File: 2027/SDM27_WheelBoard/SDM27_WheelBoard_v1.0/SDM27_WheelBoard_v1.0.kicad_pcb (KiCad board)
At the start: 4 copper layers, 38 x 22 mm, 85 parts, among them IC1 TPS2121RUXR, IC2 TPS542951RSAR, IC3 TPS2121RUXR, IC4 MLX90614ESF-BAA-000-SP, IC5 SN74LVC1G17YZPR, IC8 TCAN3403DRBRQ1, J1 WEIPU SA12 7PIN, J2 WEIPU SA6 5Pin, U1 ESP32-C5, U2 USBLC6-2SC6, Y1 Crystal_GND24

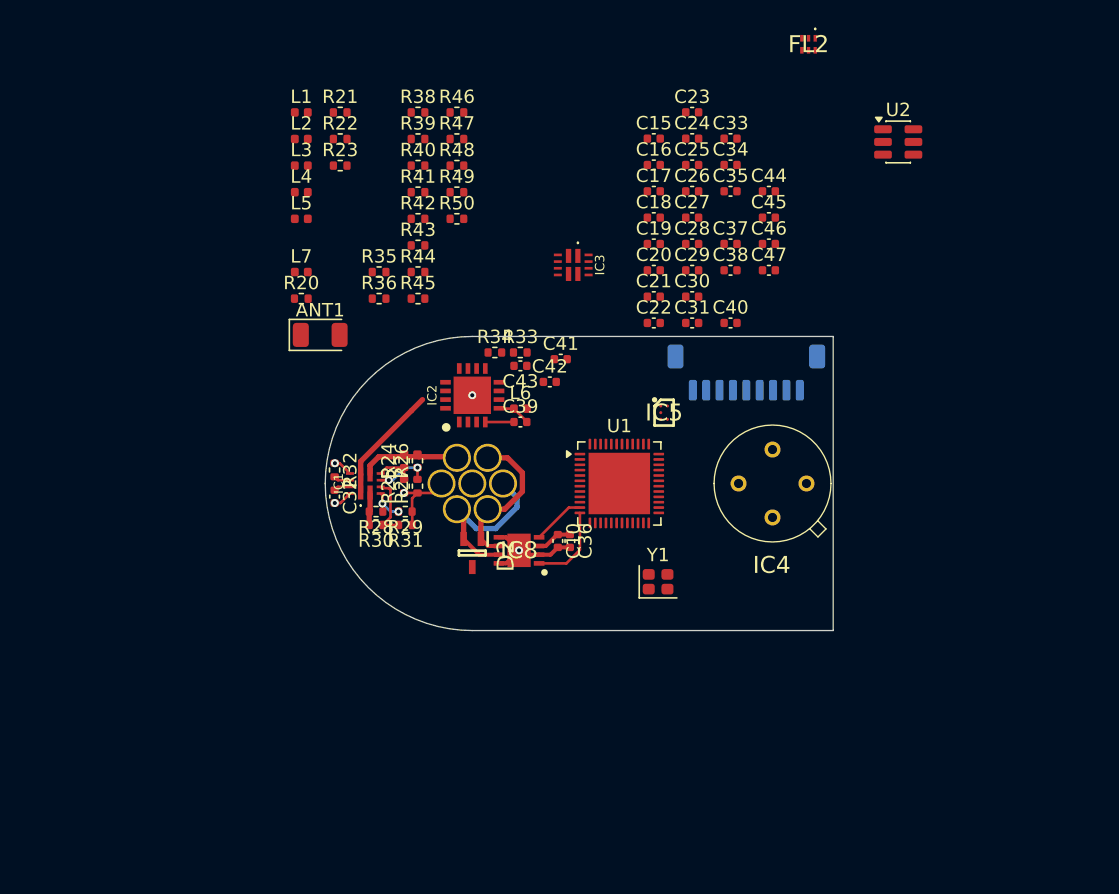
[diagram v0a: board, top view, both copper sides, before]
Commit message: board progrez 40%
its 4:30 am...
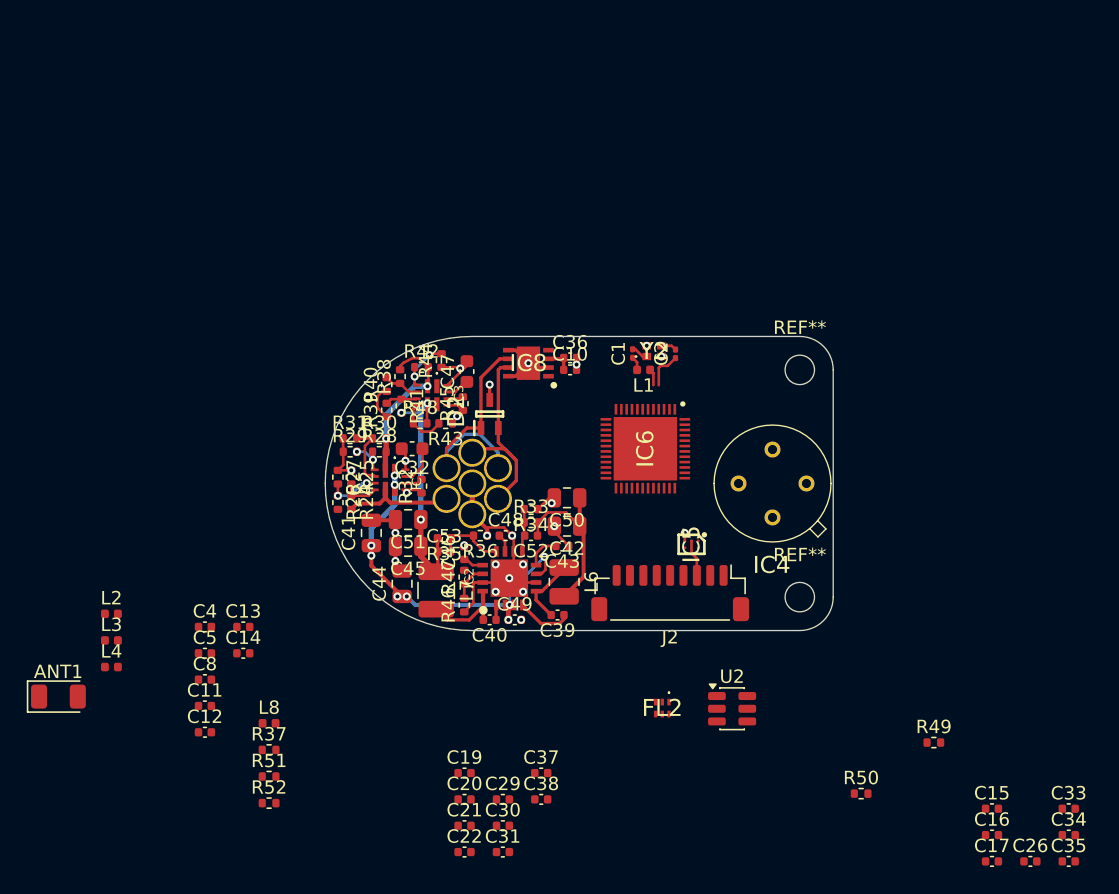
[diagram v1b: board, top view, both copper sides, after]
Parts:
- removed C18: 1uF, Capacitor_SMD:C_0402_1005Metric
- removed C23, C28: 0.1uF, Capacitor_SMD:C_0402_1005Metric
- removed C24: 2.6pF, Capacitor_SMD:C_0402_1005Metric
- removed C25: 3.0pF, Capacitor_SMD:C_0402_1005Metric
- removed C27: 10uF, Capacitor_SMD:C_0402_1005Metric
- removed L5: 2.0nH, Inductor_SMD:L_0402_1005Metric
- removed R20, R21: 4.7k, Resistor_SMD:R_0402_1005Metric
- removed R22, R23: 10k, Resistor_SMD:R_0402_1005Metric
- removed U1: ESP32-C5, Package_DFN_QFN:QFN-48-1EP_6x6mm_P0.4mm_EP4.6x4.6mm
- removed Y1: Crystal_GND24, Crystal:Crystal_SMD_2016-4Pin_2.0x1.6mm
- added C1: 12pF, Capacitor_SMD:C_0201_0603Metric, F.Cu at (123.0, 90.3)
- added C11: 3pF, Capacitor_SMD:C_0402_1005Metric, F.Cu at (91.0, 116.6)
- added C12: 0.1uF, Capacitor_SMD:C_0402_1005Metric, F.Cu at (91.0, 118.6)
- added C13: 2.6pF, Capacitor_SMD:C_0402_1005Metric, F.Cu at (93.9, 110.7)
- added C14: 10uF, Capacitor_SMD:C_0402_1005Metric, F.Cu at (93.9, 112.7)
- added C2: 12pF, Capacitor_SMD:C_0201_0603Metric, F.Cu at (126.2, 90.3)
- added C4: 0.1uF, Capacitor_SMD:C_0402_1005Metric, F.Cu at (91.0, 110.7)
- added C48: 1uF, Capacitor_SMD:C_0402_1005Metric, F.Cu at (113.5, 103.9)
- added C49: 100nF, Capacitor_SMD:C_0402_1005Metric, F.Cu at (114.2, 110.2)
- added C5: 0.1uF, Capacitor_SMD:C_0402_1005Metric, F.Cu at (91.0, 112.7)
- added C50: 22uF 10V, Capacitor_SMD:C_0805_2012Metric, F.Cu at (118.1, 101.1)
- added C51: 22uF 16V, Capacitor_SMD:C_0805_2012Metric, F.Cu at (106.2, 102.7)
- added C52: 10pF, Capacitor_SMD:C_0402_1005Metric, F.Cu at (115.4, 103.9)
- added C53: 10pF, Capacitor_SMD:C_0402_1005Metric, F.Cu at (108.9, 105.1)
- added C8: 0.1uF, Capacitor_SMD:C_0402_1005Metric, F.Cu at (91.0, 114.7)
- added IC6: ESP32-C5HF4, SDM_Misc:QFN40P600X600X90-49N-D, F.Cu at (124.0, 97.4)
- added L8: 2.0nH, Inductor_SMD:L_0402_1005Metric, F.Cu at (95.8, 117.9)
- added R37: 10k, Resistor_SMD:R_0402_1005Metric, F.Cu at (95.8, 119.9)
- added R51: 27, Resistor_SMD:R_0402_1005Metric, F.Cu at (95.8, 121.9)
- added R52: 10k, Resistor_SMD:R_0402_1005Metric, F.Cu at (95.8, 123.9)
- added REF**: MountingHole_2.2mm_M2, MountingHole:MountingHole_2.2mm_M2, F.Cu at (135.5, 91.5)
- added REF**: MountingHole_2.2mm_M2, MountingHole:MountingHole_2.2mm_M2, F.Cu at (135.5, 108.5)
- added Y2: CX1612DB48000D0FPJC1, Smart_Watch:CX1612DB48000D0FPJC1, F.Cu at (124.6, 90.1)
- C15: value 1uF -> 0.1uF
- C16: value 1uF -> 0.8pF
- C17: value 10pF -> 0.3pF
- C19: value 10uF -> 1uF
- C20: value 0.3pF -> 1uF
- C21: value 0.8pF -> 1uF
- C26: value 0.1uF -> 1uF
- C29: value 10pF -> 10uF
- C31: value 10nF -> 10uF
- C32, C47: value 1uF -> 1uF 10V 0603; footprint Capacitor_SMD:C_0402_1005Metric -> Capacitor_SMD:C_0603_1608Metric
- C41: value 100nF -> 10uF 25V; footprint Capacitor_SMD:C_0402_1005Metric -> Capacitor_SMD:C_0805_2012Metric
- C42: value 22uF -> 22uF 10V; footprint Capacitor_SMD:C_0402_1005Metric -> Capacitor_SMD:C_0805_2012Metric
- C44: value 10nF -> 10uF 25V; footprint Capacitor_SMD:C_0402_1005Metric -> Capacitor_SMD:C_0805_2012Metric
- C45: value 22nF -> 22uF 16V; footprint Capacitor_SMD:C_0402_1005Metric -> Capacitor_SMD:C_0805_2012Metric
- J2: moved to F.Cu
- L6: footprint Inductor_SMD:L_0402_1005Metric -> Inductor_SMD:L_1008_2520Metric
- L7: footprint Inductor_SMD:L_0402_1005Metric -> Inductor_SMD:L_1210_3225Metric
- R49: value 27 -> 10k
- moved C17 56.2 mm to (149.9, 128.3)
- moved C26 56.2 mm to (152.8, 128.3)
- moved C35 56.2 mm to (155.6, 128.3)
- moved C15 56.2 mm to (149.9, 124.3)
- moved C16 56.2 mm to (149.9, 126.3)
- moved C33 56.2 mm to (155.6, 124.3)
- moved C34 56.2 mm to (155.6, 126.3)
- moved R49 54.5 mm to (145.5, 119.4)
- moved R50 52.6 mm to (140.1, 123.2)
- moved FL2 50.8 mm to (125.2, 116.8)
- moved U2 44.2 mm to (130.4, 116.8)
- moved C19 42.0 mm to (110.4, 121.7)
- moved C20 42.0 mm to (110.4, 123.6)
- moved C21 42.0 mm to (110.4, 125.6)
- moved C22 42.0 mm to (110.4, 127.6)
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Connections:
- C17 pad 1: GND -> +3.3V
- C17 pad 2: Net-(C17-Pad2) -> GND
- C19 pad 1: GND -> Net-(IC6-VDDA5)
- C19 pad 2: +3.3V -> GND
- C20 pad 1: GND -> +3.3V
- C20 pad 2: +3.3V -> GND
- C21 pad 1: GND -> Net-(IC6-CHIP_PU)
- C21 pad 2: +3.3V -> GND
- C29 pad 1: GND -> +3.3V
- C29 pad 2: Net-(U1-XTAL_N) -> GND
- IC2 pad 11: GND -> Net-(IC2-VREG5)
- L1 pad 2: Net-(C17-Pad2) -> Net-(C1-Pad1)
- R49 pad 1: Net-(U1-GPIO14/USB_D+/SDIO_DATA2) -> +3.3V
- R49 pad 2: Net-(R49-Pad2) -> Net-(IC6-CHIP_PU)
- R50 pad 1: Net-(R50-Pad1) -> Net-(IC6-GPIO14)
- R50 pad 2: Net-(U1-GPIO13/USB_D-/SDIO_DATA3) -> Net-(R50-Pad2)
- U2 pad 1: Net-(R49-Pad2) -> Net-(R50-Pad2)
- U2 pad 3: Net-(R50-Pad1) -> Net-(R51-Pad1)
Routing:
- net GND: track 18.8 -> 54.8 mm, vias 5 -> 24
- net VCC: track 8.87 -> 31.0 mm, vias 0 -> 9
- net +5V PreMUX: track 0.00 -> 19.6 mm, vias 0 -> 3
- net +3.3V: track 2.65 -> 14.9 mm
- net VBUS: track 2.45 -> 12.5 mm, vias 0 -> 2
- net Net-(IC2-SW2): track 0.00 -> 7.53 mm
- net /CAN-: track 11.6 -> 18.4 mm
- net /CAN_RTX: track 6.23 -> 0.00 mm
- net Net-(IC2-VFB2): track 0.00 -> 5.21 mm
- net Net-(IC3-CP2): track 0.00 -> 4.42 mm, vias 0 -> 2
- net /CAN_CTX: track 3.97 -> 0.00 mm
- net Net-(IC3-PR1): track 0.00 -> 3.91 mm
- net Net-(IC2-VFB1): track 0.00 -> 3.25 mm
- net Net-(IC6-XTAL_N): track 0.00 -> 2.85 mm
- net /5V_EN: track 0.00 -> 2.77 mm
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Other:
- outline, holes or cut-outs redrawn
